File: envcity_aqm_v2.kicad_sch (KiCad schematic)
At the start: 139 parts, among them IC1 DS1307ZN+, IC2 DMMT5401-7F, IC3 DMMT5401-7F, IC4 DMMT5401-7-F, IC6 ESP32-S2-SOLO-N4R2, J1 USB_B_Micro, J12 Conn_01x06_Male, J13 Conn_01x06_Male, J14 Conn_01x08_Pin, J15 Conn_01x02_Male, J16 Conn_01x02_Male, J2 Screw_Terminal_01x02, J3 Screw_Terminal_01x02, J6 Conn_01x04_Male, J7 Conn_01x06_Pin, J8 503398-1892, Q1 DMG2301L / DMP2045U, Q2 DMG2301L / DMP2045U, Q3 DMG2301L, Q4 DMG2301L, Q5 DMG2301L / DMP2045U, Q6 DMG2301L, Q7 DMN10H220L, Q8 DMN10H220L, SW1 BOOT, SW1 RESET, U1 TP4056, U10 RFM95W-915S2, U11 ADS1115IDGS, U12 TPS54202DDC, U2 USBLC6-2SC6, U3 MT3608, U4 SHT30-DIS, U5 LM2596S-5, U6 AP2112K-3.3, U7 DHT11, U8 AP2112K-3.3, U9 74HC4067DB, Y2 AB26TRB

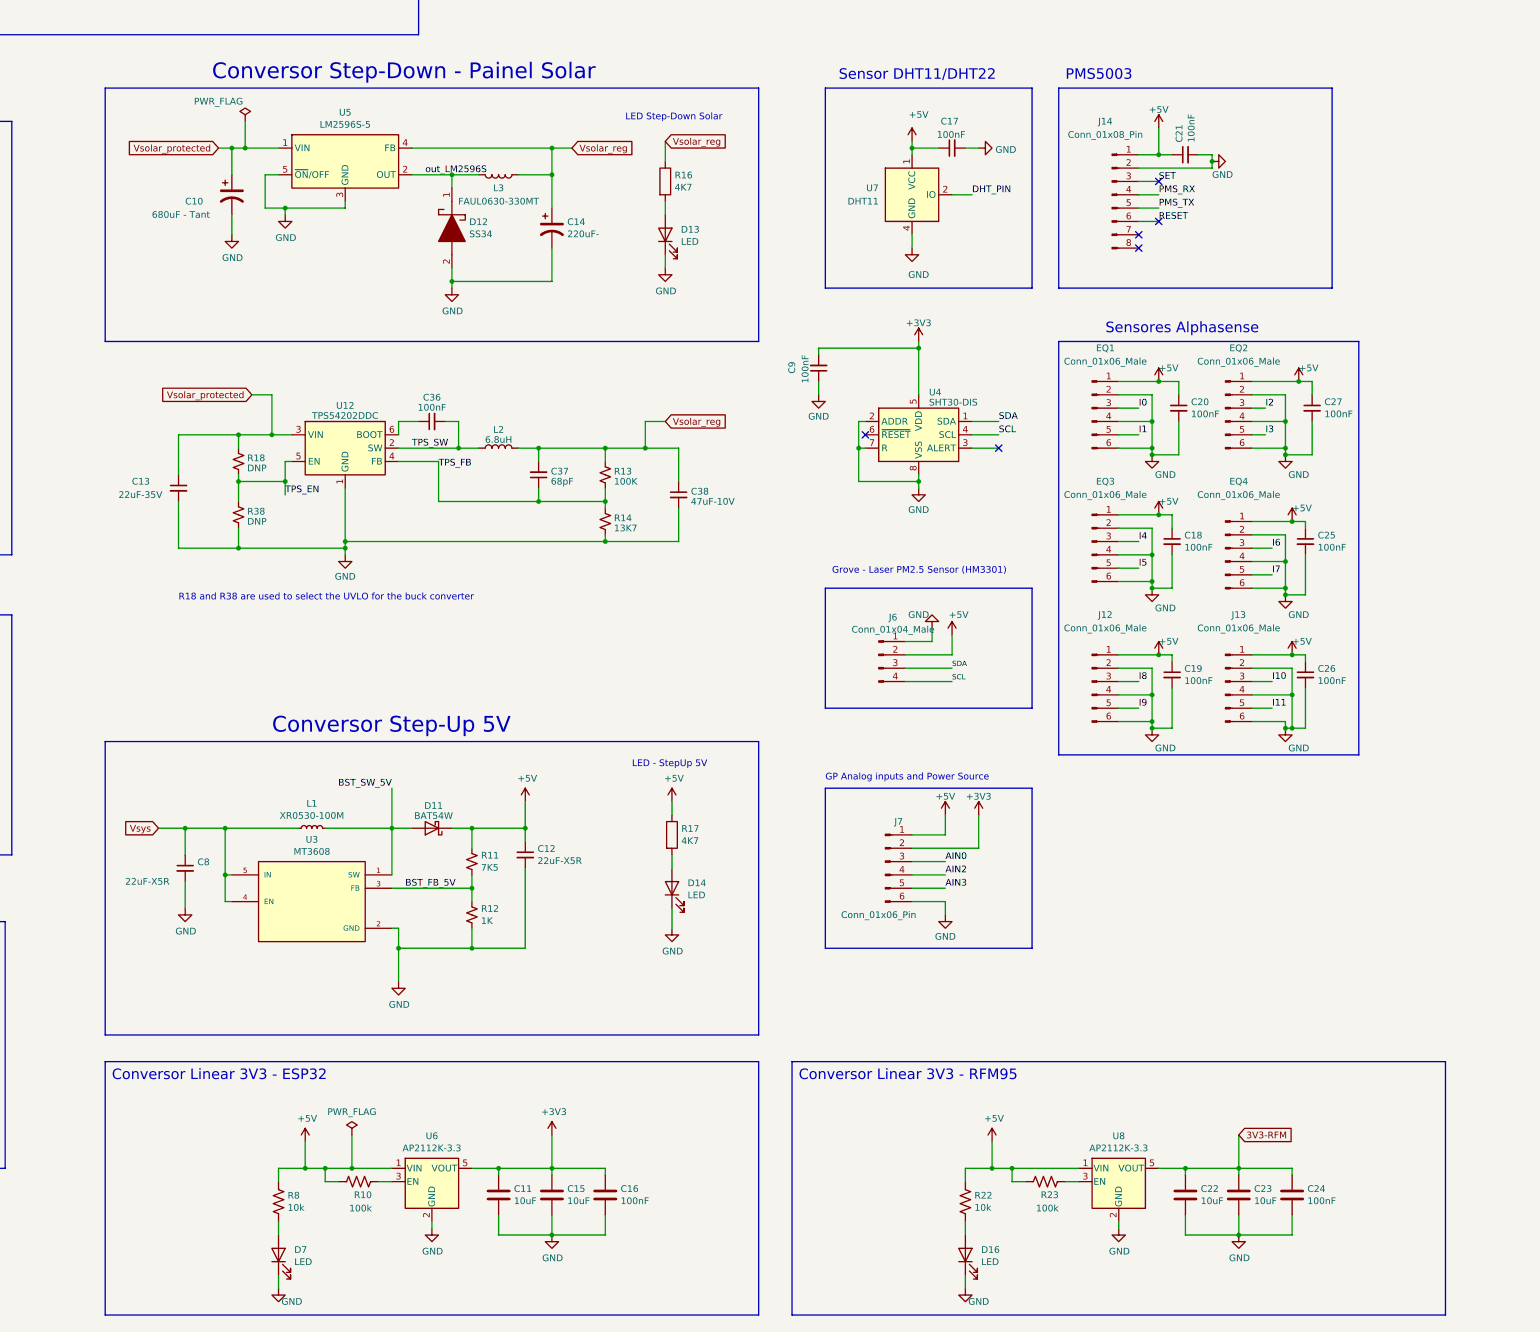
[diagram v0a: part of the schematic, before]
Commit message: add novo conversor
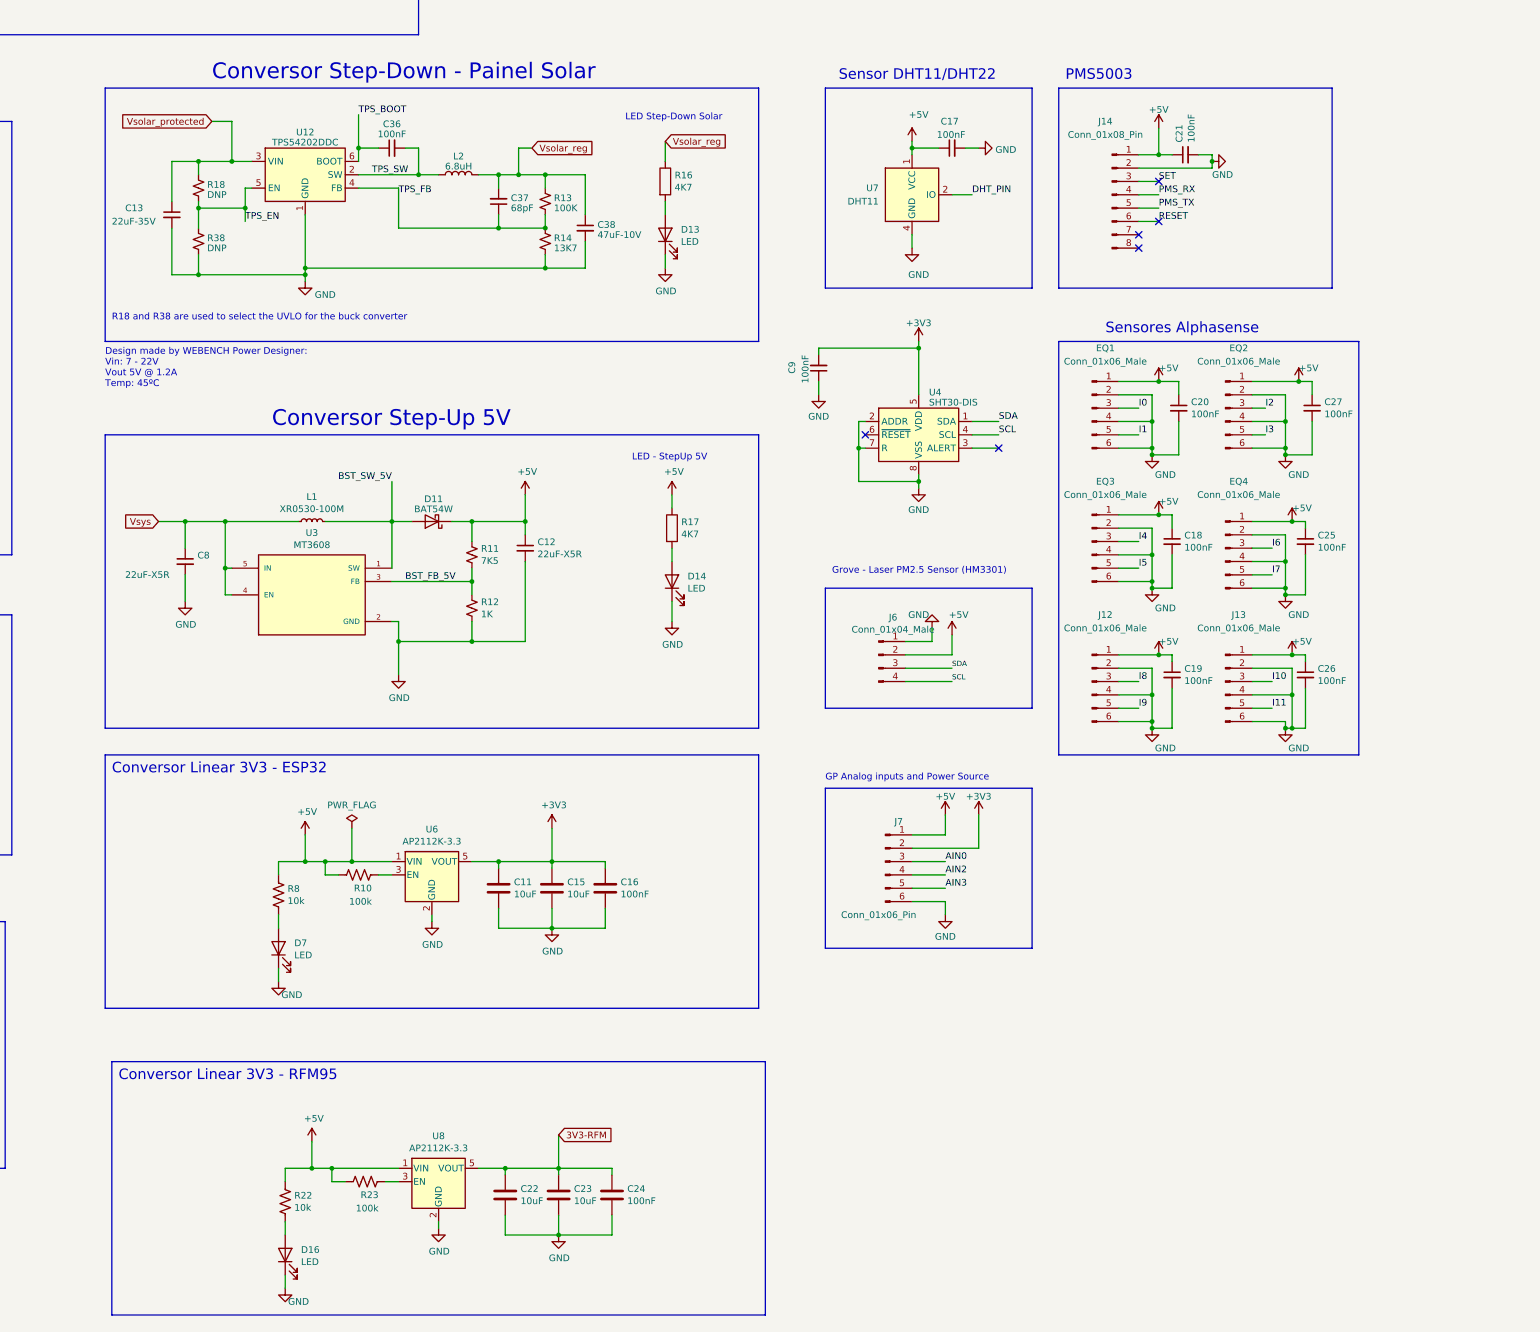
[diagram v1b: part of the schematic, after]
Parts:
- removed C10: 680uF - Tant, Capacitor_Tantalum_SMD:CP_EIA-7343-15_Kemet-W_Pad2.25x2.55mm_HandSolder, symbol envcity_aqm_v2-rescue:CP1-Device
- removed C14: 220uF-, Capacitor_Tantalum_SMD:CP_EIA-7343-15_Kemet-W_Pad2.25x2.55mm_HandSolder, symbol envcity_aqm_v2-rescue:CP1-Device
- removed D12: SS34, Diode_SMD:D_SMB, symbol envcity_aqm_v2-rescue:SS34-SamacSys_Parts
- removed L3: FAUL0630-330MT, FDSD0630-H-1R0M_P3:IND_FDSD0630-H-1R0M=P3, symbol Device:L
- removed U5: LM2596S-5, Package_TO_SOT_SMD:TO-263-5_TabPin3, symbol Regulator_Switching:LM2596S-5
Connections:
- net TPS_BOOT: now reaches C36.1, U12.6 (BOOT)
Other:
- note added: "Design made by WEBENCH Power Designer: Vin: 7 - 22V Vout 5V @ 1.2A Temp: 45ºC"
- moved on the sheet: C11, C12, C13, C15, C16, C22, C23, C24, C36, C37, C38, C8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
